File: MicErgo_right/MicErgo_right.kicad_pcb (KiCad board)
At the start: 2 copper layers, 179.9 x 110.5 mm, 82 parts, among them J1 MJ-4PP-9_BL_kai, SW00 SW_Push, SW1 SW_Push, SW10 SW_Push, SW11 SW_Push, SW12 SW_Push, SW13 SW_Push, SW14 SW_Push, SW15 SW_Push, SW16 SW_Push, SW17 SW_Push, SW18 SW_Push, SW19 SW_Push, SW2 SW_Push, SW20 SW_Push, SW21 SW_Push, SW22 SW_Push, SW23 SW_Push, SW24 SW_Push, SW25 SW_Push, SW26 SW_Push, SW27 SW_Push, SW28 SW_Push, SW29 SW_Push, SW3 SW_Push, SW30 SW_Push, SW31 SW_Push, SW32 SW_Push, SW33 SW_Push, SW34 SW_Push, SW35 SW_Push, SW4 SW_Push, SW5 SW_Push, SW6 SW_Push, SW7 SW_Push, SW8 SW_Push, SW9 SW_Push, U1 ProMicro

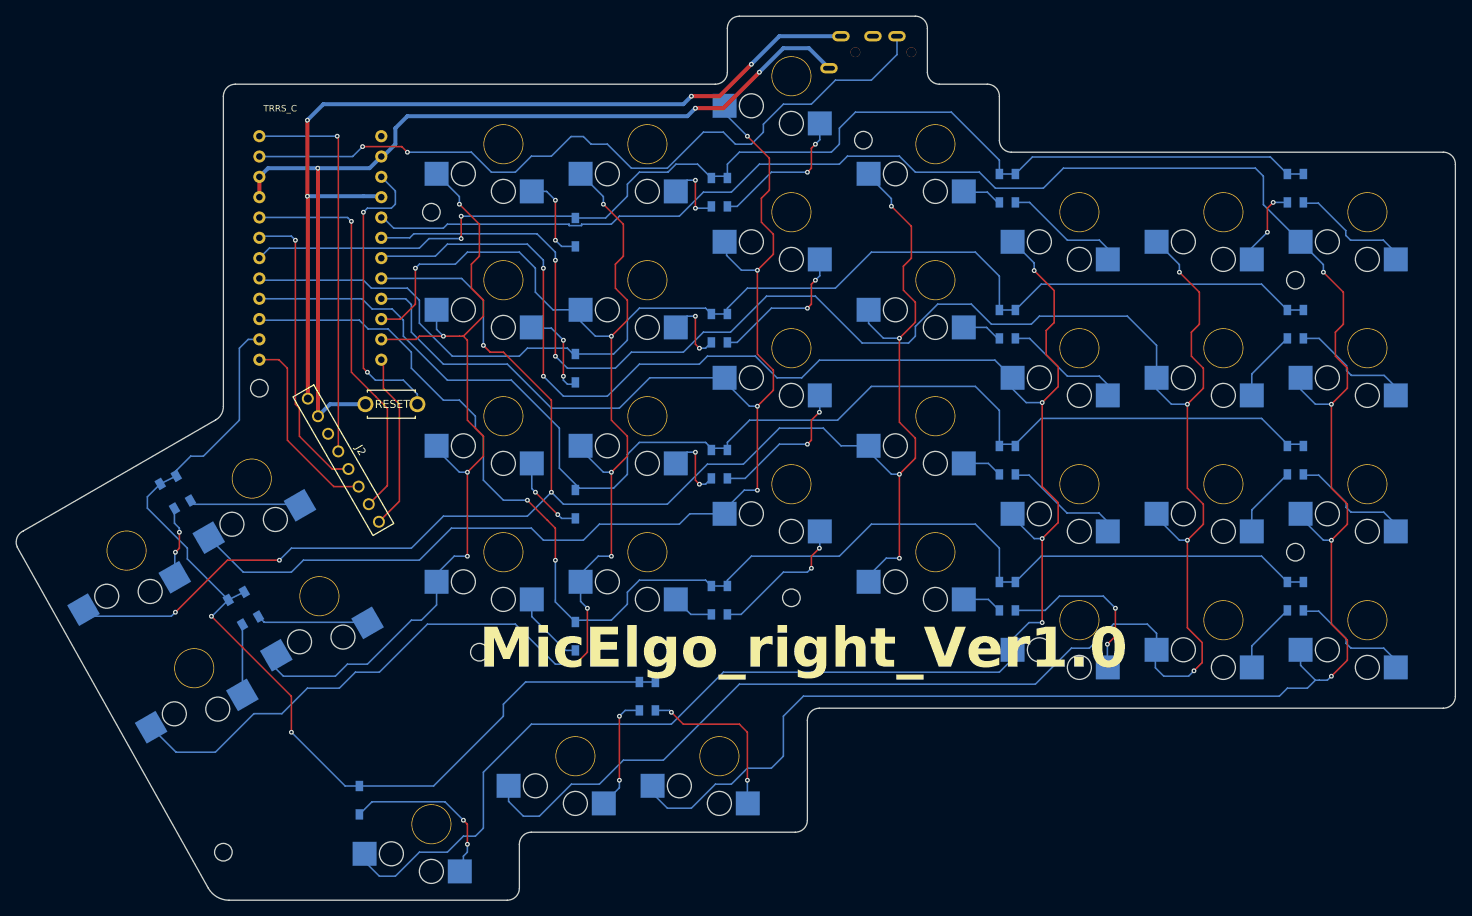
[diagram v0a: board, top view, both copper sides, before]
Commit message: Add files via upload
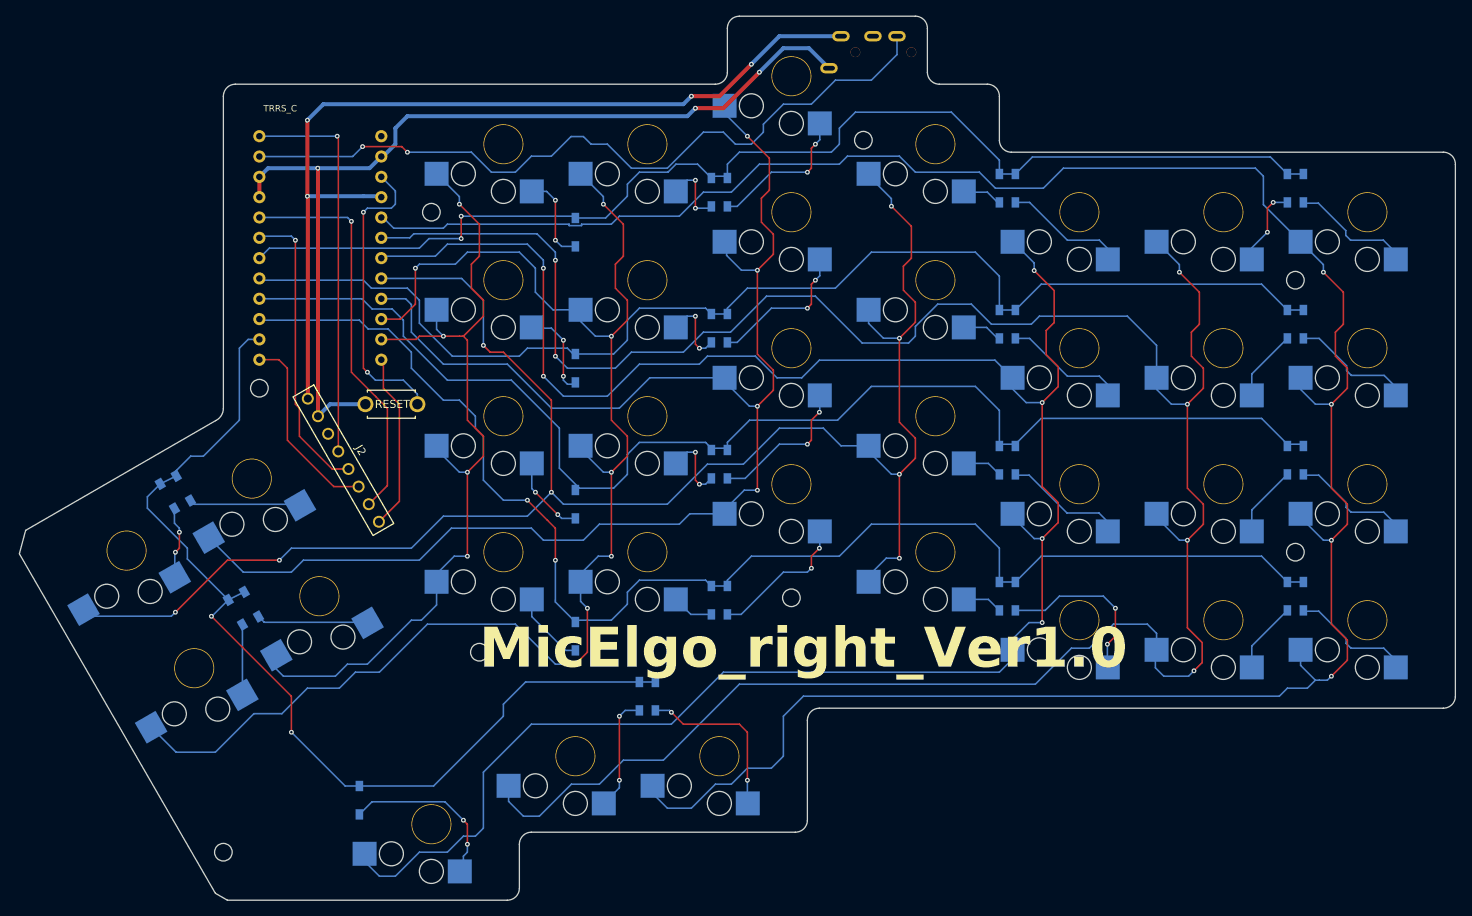
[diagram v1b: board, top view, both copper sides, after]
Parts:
- D1, D10, D11, D12, D13, D14, D15, D16, D17, D18, D19, D2, D20, D21, D22, D23, D24, D25, D26, D27, D28, D29, D3, D30, D31, D32, D33, D34, D35, D4, D5, D6, D7, D8, D9: footprint my_foot:Diode_SMD_top -> my-foot:Diode_SMD_top
- J1: value MJ-4PP-9_BL_kai -> TRRS_MJ-4PP-9
- J2: footprint my_foot:PMW3360 -> my-foot:PMW3360
- SW1, SW10, SW11, SW12, SW13, SW14, SW15, SW16, SW17, SW18, SW19, SW2, SW20, SW21, SW22, SW23, SW24, SW25, SW26, SW27, SW28, SW29, SW3, SW30, SW31, SW32, SW33, SW34, SW35, SW4, SW5, SW6, SW7, SW8, SW9: footprint my_foot:Choc_v2_Hotswap_1u_Narrow -> my-foot:Choc_v2_Hotswap_1u_Narrow
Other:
- board size 179.9 x 110.5 mm -> 179.5 x 110.5 mm
